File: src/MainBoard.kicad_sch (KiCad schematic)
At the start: 75 parts, among them J10 1217080-1, J11 1217080-1, J12 1217080-1, J13 1217080-1, J14 1217080-1, J15 1217080-1, J16 1217080-1, J4 MiniFit_2x08_F, J5 1217080-1, J6 1217080-1, J7 1217080-1, J8 1217080-1, J9 1217080-1, K1 RAYEX-L90S, K2 LR2A-12W, K3 LR2A-12W, Q1 BC547, Q10 2N7002, Q3 2N7002, Q4 2N7002, Q5 2N7002, Q6 2N7002, Q7 BC547, Q8 BC557, Q9 2N7002, U1 ATtiny85-20P

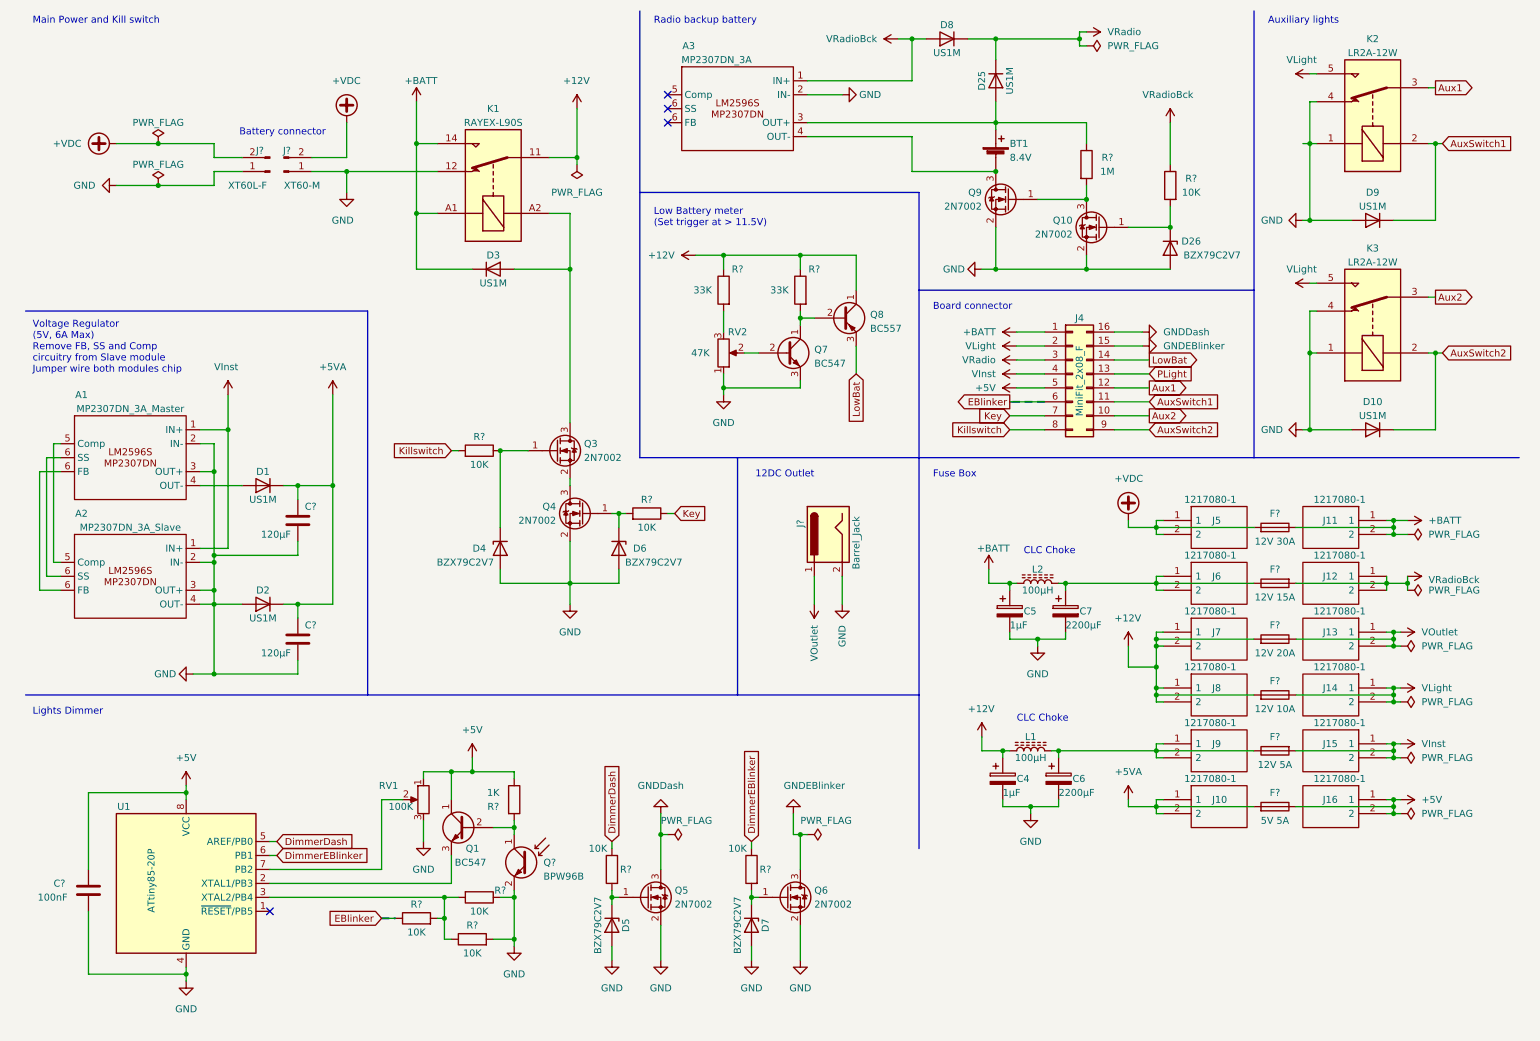
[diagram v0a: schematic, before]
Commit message: Update schematics
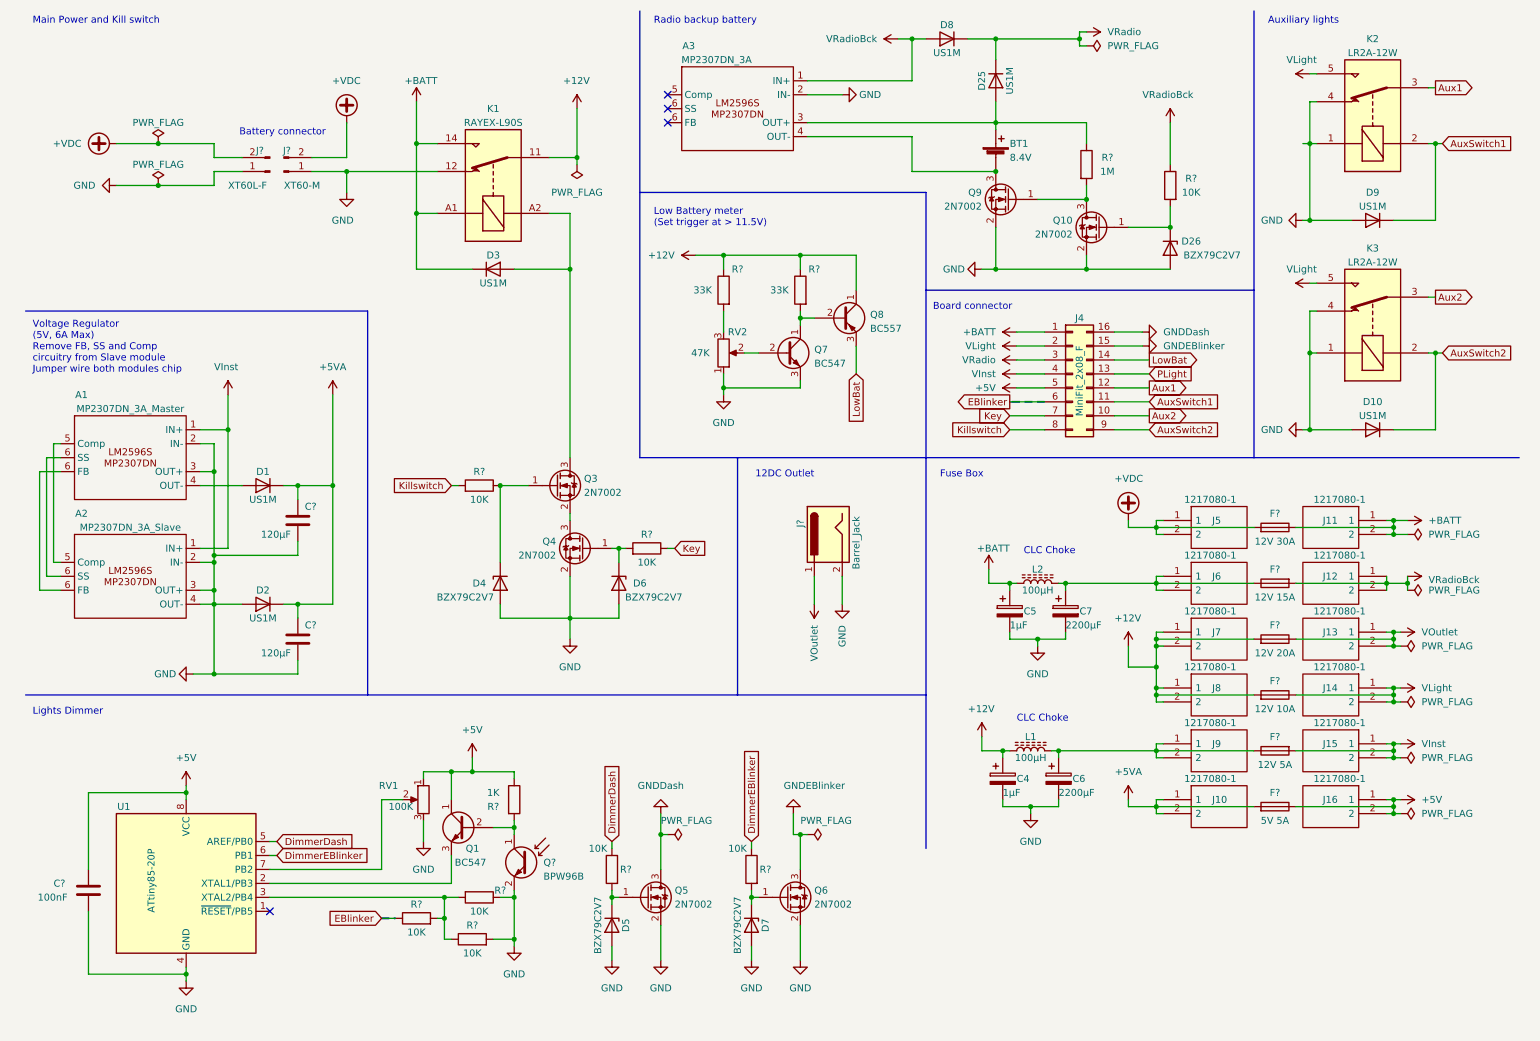
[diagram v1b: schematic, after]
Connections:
- new net: A1.6 (SS), A2.6 (SS)
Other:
- moved on the sheet: D4, D6, Q3, Q4, R?

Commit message: update Schematics
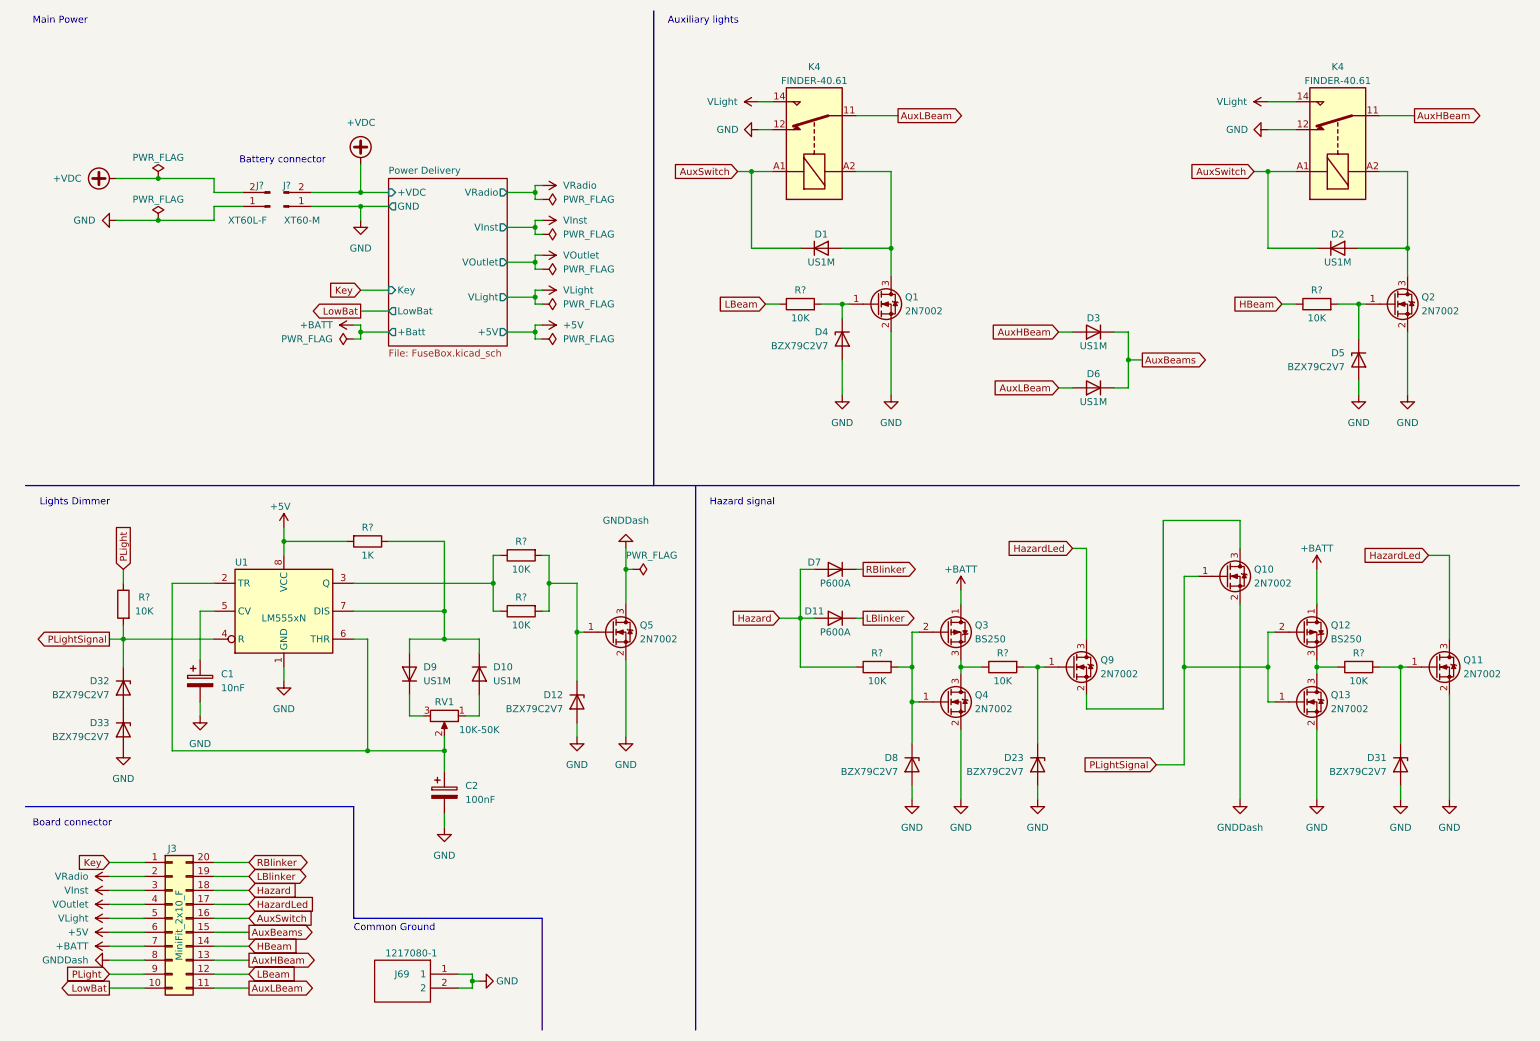
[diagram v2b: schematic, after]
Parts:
- removed A1: MP2307DN_3A_Master, symbol Modules:MP2307DN_3A
- removed A2: MP2307DN_3A_Slave, symbol Modules:MP2307DN_3A
- removed A3: MP2307DN_3A, symbol Modules:MP2307DN_3A
- removed BT1: 8.4V, symbol Device:Battery_Cell
- removed C4, C5: 1µF, symbol Device:C_Polarized
- removed C6, C7: 2200µF, symbol Device:C_Polarized
- removed C? (x2): 120µF, Capacitor_THT:C_Disc_D5.0mm_W2.5mm_P5.00mm, symbol Device:C
- removed C?: 100nF, Capacitor_THT:C_Disc_D5.0mm_W2.5mm_P5.00mm, symbol Device:C
- removed D25, D8: US1M, Diode_SMD:D_SMA, symbol Diode:US1M
- removed D26, D6, D7: BZX79C2V7, Diode_SMD:D_MiniMELF, symbol Diode:BZV55C2V7
- removed F?: 12V 5A, symbol Device:Fuse
- removed F?: 12V 30A, symbol Device:Fuse
- removed F?: 12V 20A, symbol Device:Fuse
- removed F?: 12V 15A, symbol Device:Fuse
- removed F?: 12V 10A, symbol Device:Fuse
- removed F?: 5V 5A, symbol Device:Fuse
- removed J10, J11, J12, J13, J14, J15, J16, J5, J6, J7, J8, J9: 1217080-1, 1217080-1, symbol SamacSys_Parts:1217080-1
- removed J4: MiniFit_2x08_F, Connector_Molex:Molex_Mini-Fit_Jr_5566-16A_2x08_P4.20mm_Vertical, symbol Connector_Generic:Conn_02x08_Counter_Clockwise
- removed J?: Barrel_Jack, Connector_BarrelJack:BarrelJack_CUI_PJ-063AH_Horizontal, symbol Connector:Barrel_Jack
- removed J?: XT60-M, Connector_AMASS:AMASS_XT60PW-M_1x02_P7.20mm_Horizontal, symbol Connector:Conn_01x02_Pin
- removed J?: XT60L-F, Connector_AMASS:AMASS_XT60-M_1x02_P7.20mm_Vertical, symbol Connector:Conn_01x02_Pin
- removed K1: RAYEX-L90S, Relay_THT:Relay_SPDT_RAYEX-L90S, symbol Relay:RAYEX-L90S
- removed K2: LR2A-12W, SamacSys_Parts:AZ9431CH12DE, symbol Local Components:LR2A-12W
- removed K3: LR2A-12W, Relay_THT:Relay_SPDT_Finder_36.11, symbol Local Components:LR2A-12W
- removed L1, L2: 100µH, symbol Device:L_Ferrite
- removed Q1, Q7: BC547, Package_TO_SOT_THT:TO-92_Inline, symbol Transistor_BJT:BC547
- removed Q3, Q6: 2N7002, Package_TO_SOT_SMD:SOT-23, symbol Transistor_FET:2N7002
- removed Q8: BC557, Package_TO_SOT_THT:TO-92_Inline, symbol Transistor_BJT:BC557
- removed Q?: BPW96B, LED_THT:LED_D5.0mm, symbol Device:Q_Photo_NPN
- removed R? (x7): 10K, Resistor_SMD:R_1206_3216Metric_Pad1.30x1.75mm_HandSolder, symbol Device:R
- removed R? (x2): 33K, Resistor_SMD:R_1206_3216Metric_Pad1.30x1.75mm_HandSolder, symbol Device:R
- removed R?: 1K, Resistor_THT:R_Axial_DIN0204_L3.6mm_D1.6mm_P5.08mm_Horizontal, symbol Device:R
- removed R?: 1M, Resistor_SMD:R_1206_3216Metric_Pad1.30x1.75mm_HandSolder, symbol Device:R
- removed RV2: 47K, symbol Device:R_Potentiometer
- removed U1: ATtiny85-20P, Package_DIP:DIP-8_W7.62mm, symbol MCU_Microchip_ATtiny:ATtiny85-20P
- added C1: 10nF, symbol Device:C_Polarized
- added C2: 100nF, symbol Device:C_Polarized
- added D11, D7: P600A, Diode_THT:D_P600_R-6_P12.70mm_Horizontal, symbol Device:D
- added D23, D31, D32, D33, D5, D8: BZX79C2V7, Diode_SMD:D_MiniMELF, symbol Diode:BZV55C2V7
- added D6: US1M, Diode_SMD:D_SMA, symbol Diode:US1M
- added J3: MiniFit_2x10_F, symbol Connector_Generic:Conn_02x10_Counter_Clockwise
- added J69: 1217080-1, 1217080-1, symbol SamacSys_Parts:1217080-1
- added J?: XT60-M, Connector_AMASS:AMASS_XT60PW-M_1x02_P7.20mm_Horizontal, symbol Connector:Conn_01x02_Pin
- added J?: XT60L-F, Connector_AMASS:AMASS_XT60-M_1x02_P7.20mm_Vertical, symbol Connector:Conn_01x02_Pin
- added K4 (x2): FINDER-40.61, Relay_THT:Relay_DPDT_Finder_40.52, symbol Relay:FINDER-40.51
- added Q1, Q11, Q13, Q2: 2N7002, Package_TO_SOT_SMD:SOT-23, symbol Transistor_FET:2N7002
- added Q12, Q3: BS250, Package_TO_SOT_THT:TO-92_Inline, symbol Transistor_FET:BS250
- added R? (x7): 10K, Resistor_SMD:R_1206_3216Metric_Pad1.30x1.75mm_HandSolder, symbol Device:R
- added R?: 1K, Resistor_SMD:R_1206_3216Metric_Pad1.30x1.75mm_HandSolder, symbol Device:R
- added U1: LM555xN, Package_DIP:DIP-8_W7.62mm, symbol Timer:LM555xN
- RV1: value 100K -> 10K-50K
- renumbered D5 to D12
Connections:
- net +5V: now also J3.6 (Pin_6), R?.2, U1.8 (VCC); no longer RV1.1
- net +BATT: now also J3.7 (Pin_7), Q12.1 (D), Q3.1 (D); no longer D3.1 (K)
- net +VDC: now also J?.2 (Pin_2), J?.2 (Pin_2)
- net GND: now also C1.2, C2.2, D23.2 (A), D31.2 (A), D33.2 (A), D5.2 (A), D8.2 (A), J69.1, J69.2, J?.1 (Pin_1), J?.1 (Pin_1), K4.12, K4.12, Q1.2 (S), Q11.2 (S), Q13.2 (S), Q2.2 (S), U1.1 (GND); no longer D10.2 (A), D2.2 (A), D9.2 (A), Q10.2 (S), Q9.2 (S), RV1.3
- net GNDDash: now also Q10.2 (S), J3.8 (Pin_8)
- net Key: now also J3.1 (Pin_1)
- net LowBat: now also J3.10 (Pin_10)
- net PLight: now also J3.9 (Pin_9), R?.1
- net VInst: now also J3.3 (Pin_3)
- net VLight: now also J3.5 (Pin_5), K4.14, K4.14
- net VOutlet: now also J3.4 (Pin_4)
- net VRadio: now also J3.2 (Pin_2)
- net at Q4.1 (G): now also D8.1 (K), Q3.2 (G), R?.2
- net at Q4.3 (D): now also Q3.3 (S), R?.1
- net PLightSignal: now reaches Q10.1 (G)
- net PLightSignal: now also D32.1 (K), Q12.2 (G), Q13.1 (G), R?.2, U1.4 (R)
- net at Q9.1 (G): now also D23.1 (K), R?.2; no longer Q10.3 (D)
- net AuxHBeam: now reaches D3.2 (A)
- net AuxHBeam: now also J3.13 (Pin_13), K4.11
- net at D12.1 (K), Q5.1 (G), R?.2: now also R?.2
- net at RV1.2: now also C2.1, U1.2 (TR), U1.6 (THR)
- net at D4.1 (K): now also Q1.1 (G), R?.2
- net at D1.2 (A): now also K4.A2, Q1.3 (D)
- net HazardLed: now reaches Q9.3 (D)
- net HazardLed: now also J3.17 (Pin_17), Q11.3 (D)
- net +5VA renamed AuxSwitch
- net AuxSwitch: now also J3.16 (Pin_16), K4.A1, K4.A1
- net AuxSwitch1: no longer names the net of D9.1 (K)
- net AuxSwitch1: now also RV1.3
- net AuxSwitch2: no longer names the net of D10.1 (K)
- net AuxSwitch2: now also D9.2 (A), R?.1, U1.7 (DIS)
- net DimmerDash: no longer names the net of R?.1
- net DimmerDash: now also R?.1, U1.3 (Q)
- new net: D2.2 (A), K4.A2, Q2.3 (D)
- new net: D32.2 (A), D33.1 (K)
- new net: Q12.3 (S), Q13.3 (D), R?.1
- new net: D31.1 (K), Q11.1 (G), R?.2
- new net: D5.1 (K), Q2.1 (G), R?.2
- new net: C1.1, U1.5 (CV)
- new net: D10.2 (A), RV1.1
- new net: Q10.3 (D), Q9.2 (S)
- new net AuxBeams: D3.1 (K), D6.1 (K), J3.15 (Pin_15)
- new net AuxLBeam: D6.2 (A), J3.11 (Pin_11), K4.11
- new net HBeam: J3.14 (Pin_14), R?.1
- new net Hazard: D11.2 (A), D7.2 (A), J3.18 (Pin_18), R?.1
- new net LBeam: J3.12 (Pin_12), R?.1
- new net LBlinker: D11.1 (K), J3.19 (Pin_19)
- new net RBlinker: D7.1 (K), J3.20 (Pin_20)
- no-connect marks 4 -> 0
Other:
- added sheet Power Delivery (FuseBox.kicad_sch)
- note added: "Common Ground"
- note added: "Hazard signal"
- note added: "Main Power"
- note removed: "12DC Outlet"
- note removed: "CLC Choke"
- note removed: "Fuse Box"
- note removed: "Low Battery meter (Set trigger at > 11.5V)"
- note removed: "Main Power and Kill switch"
- note removed: "Radio backup battery"
- note removed: "Voltage Regulator (5V, 6A Max) Remove FB, SS and Comp circuitry from Slave module Jumper wire both modules chip"
- moved on the sheet: D12, Q5, R?
